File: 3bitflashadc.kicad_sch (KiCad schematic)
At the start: 31 parts, among them U1 LM339, U2 LM339, U3 74148, U4 74LS04, U5 7447

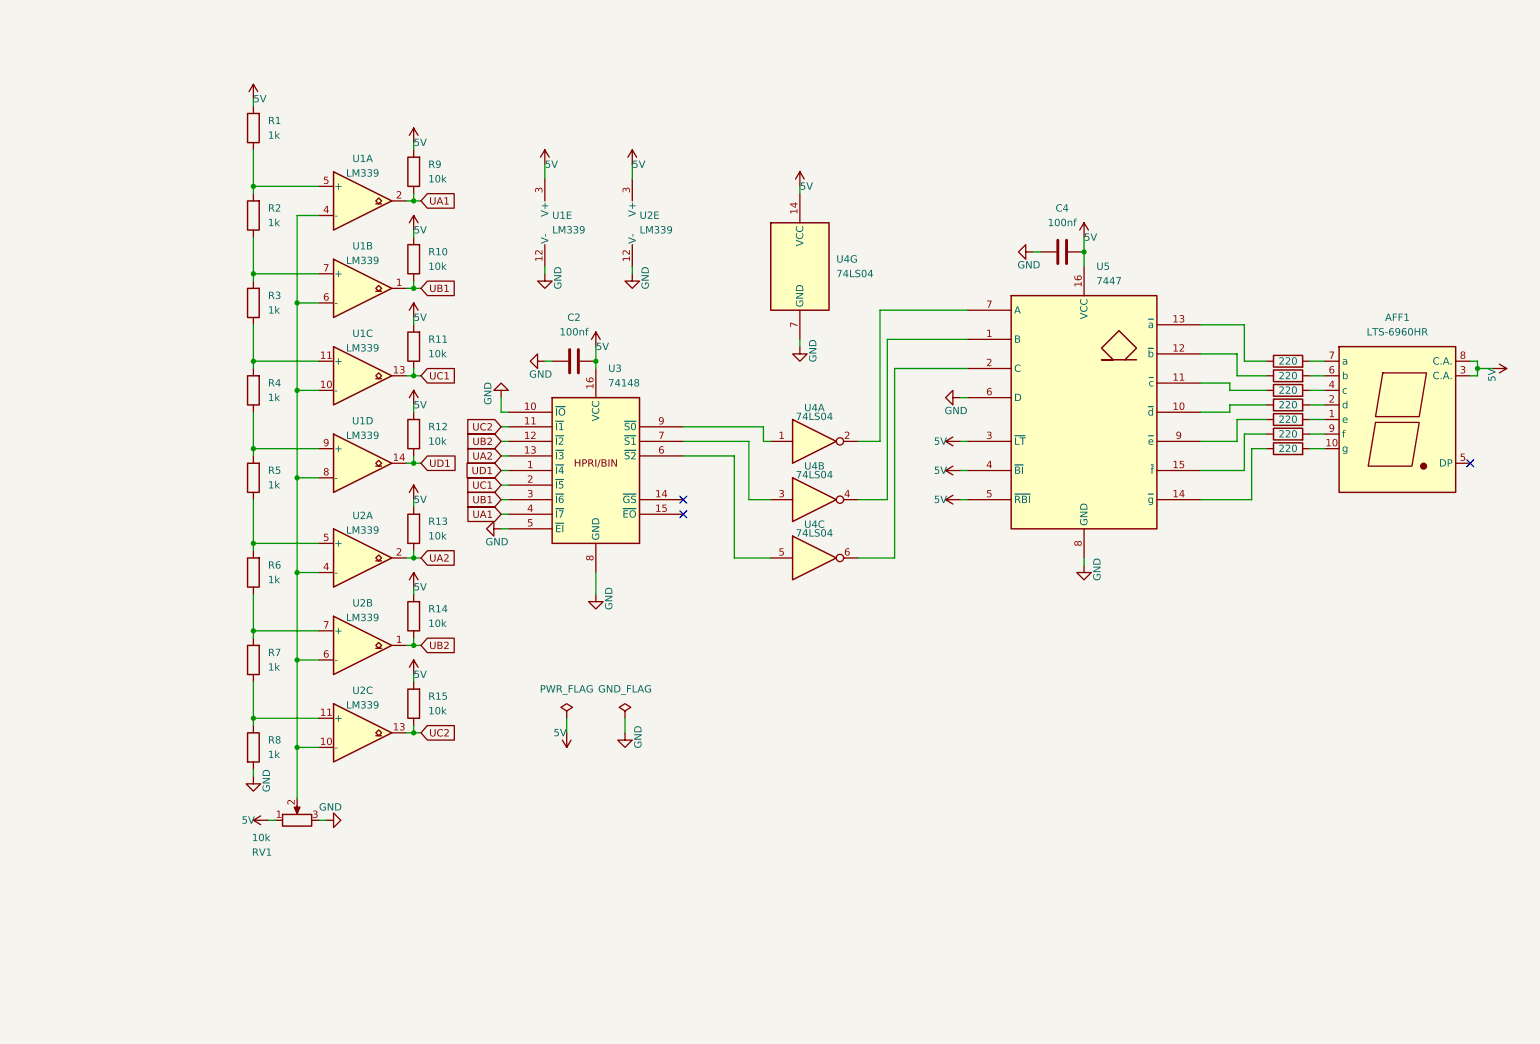
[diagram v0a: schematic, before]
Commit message: Completed schematic, still need to be inspected
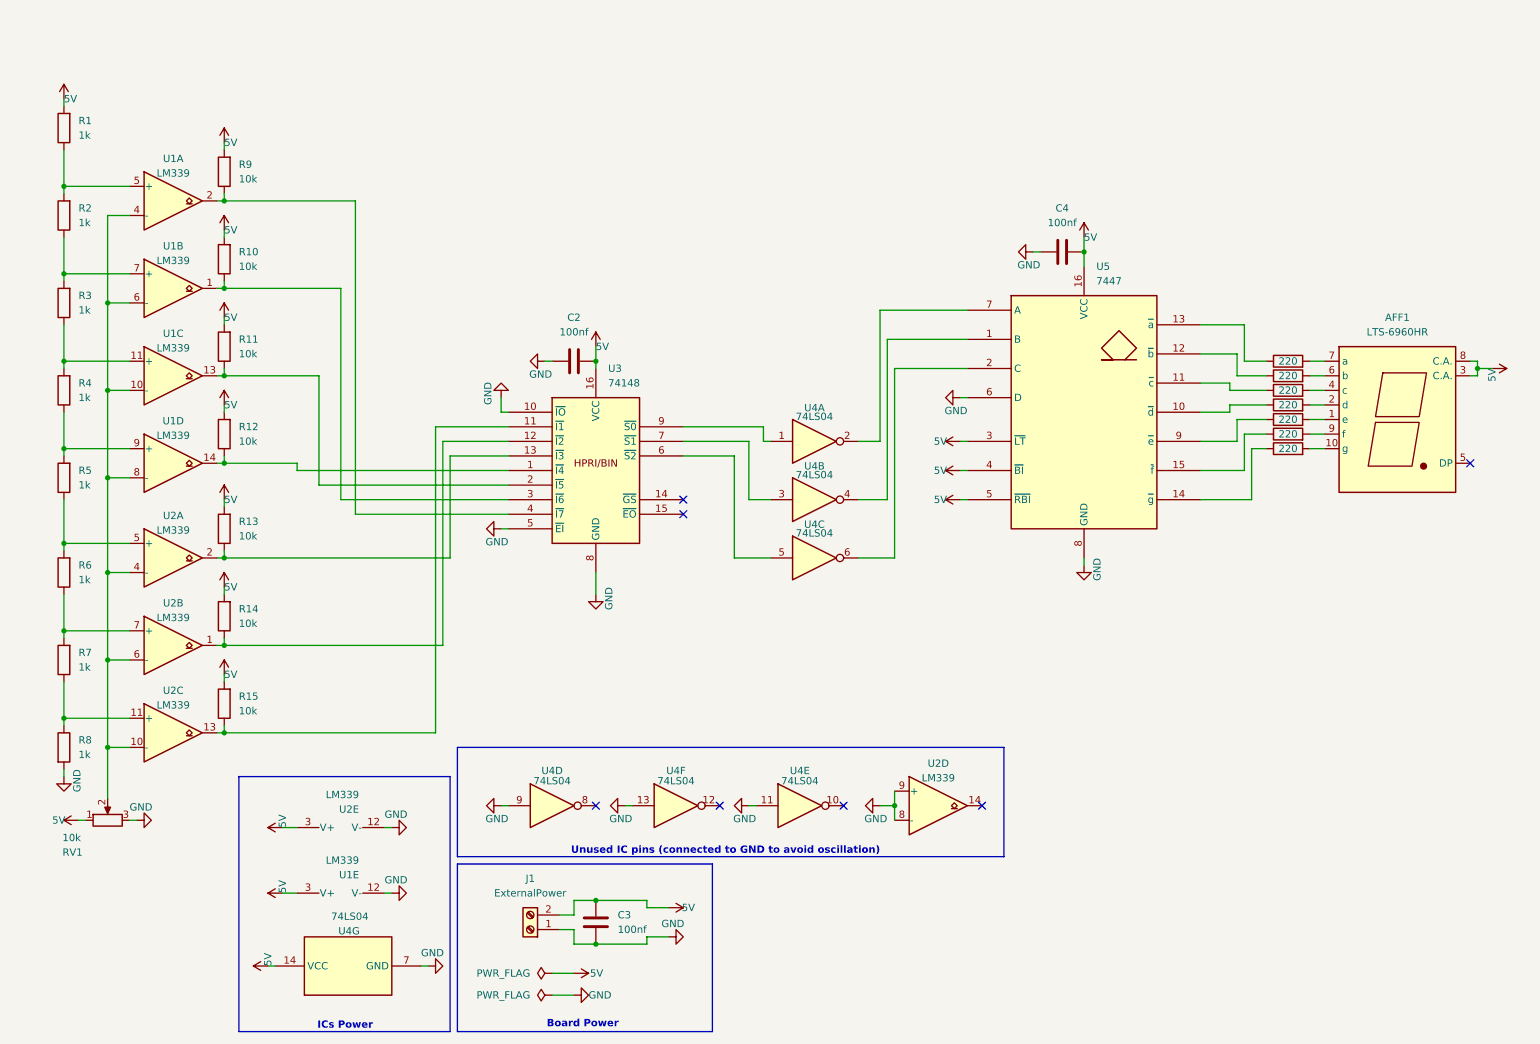
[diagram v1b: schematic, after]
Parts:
- added C3: 100nf, Capacitor_THT:C_Disc_D3.4mm_W2.1mm_P2.50mm, symbol Device:C
- added J1: ExternalPower, TerminalBlock:TerminalBlock_MaiXu_MX126-5.0-02P_1x02_P5.00mm, symbol Connector:Screw_Terminal_01x02
- added unit 4 of U2
- added unit 4 of U4
- added unit 6 of U4
- added unit 5 of U4
- U3: footprint Package_DIP:CERDIP-14_W7.62mm_SideBrazed_LongPads -> Package_DIP:CERDIP-16_W7.62mm_SideBrazed_LongPads
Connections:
- net 5V: now also C3.2, J1.2 (Pin_2)
- net GND: now also C3.1, J1.1 (Pin_1), U2.8 (-), U2.9 (+), U4.11, U4.13, U4.9
- net UA1: no longer names the net of R9.1, U1.2, U3.4 (~{I7})
- net UA2: no longer names the net of R13.1, U2.2, U3.13 (~{I3})
- net UB1: no longer names the net of R10.1, U1.1, U3.3 (~{I6})
- net UB2: no longer names the net of R14.1, U2.1, U3.12 (~{I2})
- net UC1: no longer names the net of R11.1, U1.13, U3.2 (~{I5})
- net UC2: no longer names the net of R15.1, U2.13, U3.11 (~{I1})
- net UD1: no longer names the net of R12.1, U1.14, U3.1 (~{I4})
- no-connect marks 3 -> 7
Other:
- note added: "Board Power"
- note added: "ICs Power"
- note added: "Unused IC pins (connected to GND to avoid oscillation)"
- moved on the sheet: R1, R10, R11, R12, R13, R14, R15, R2, R3, R4, R5, R6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

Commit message: Done with the schematic and working with the PCB routing
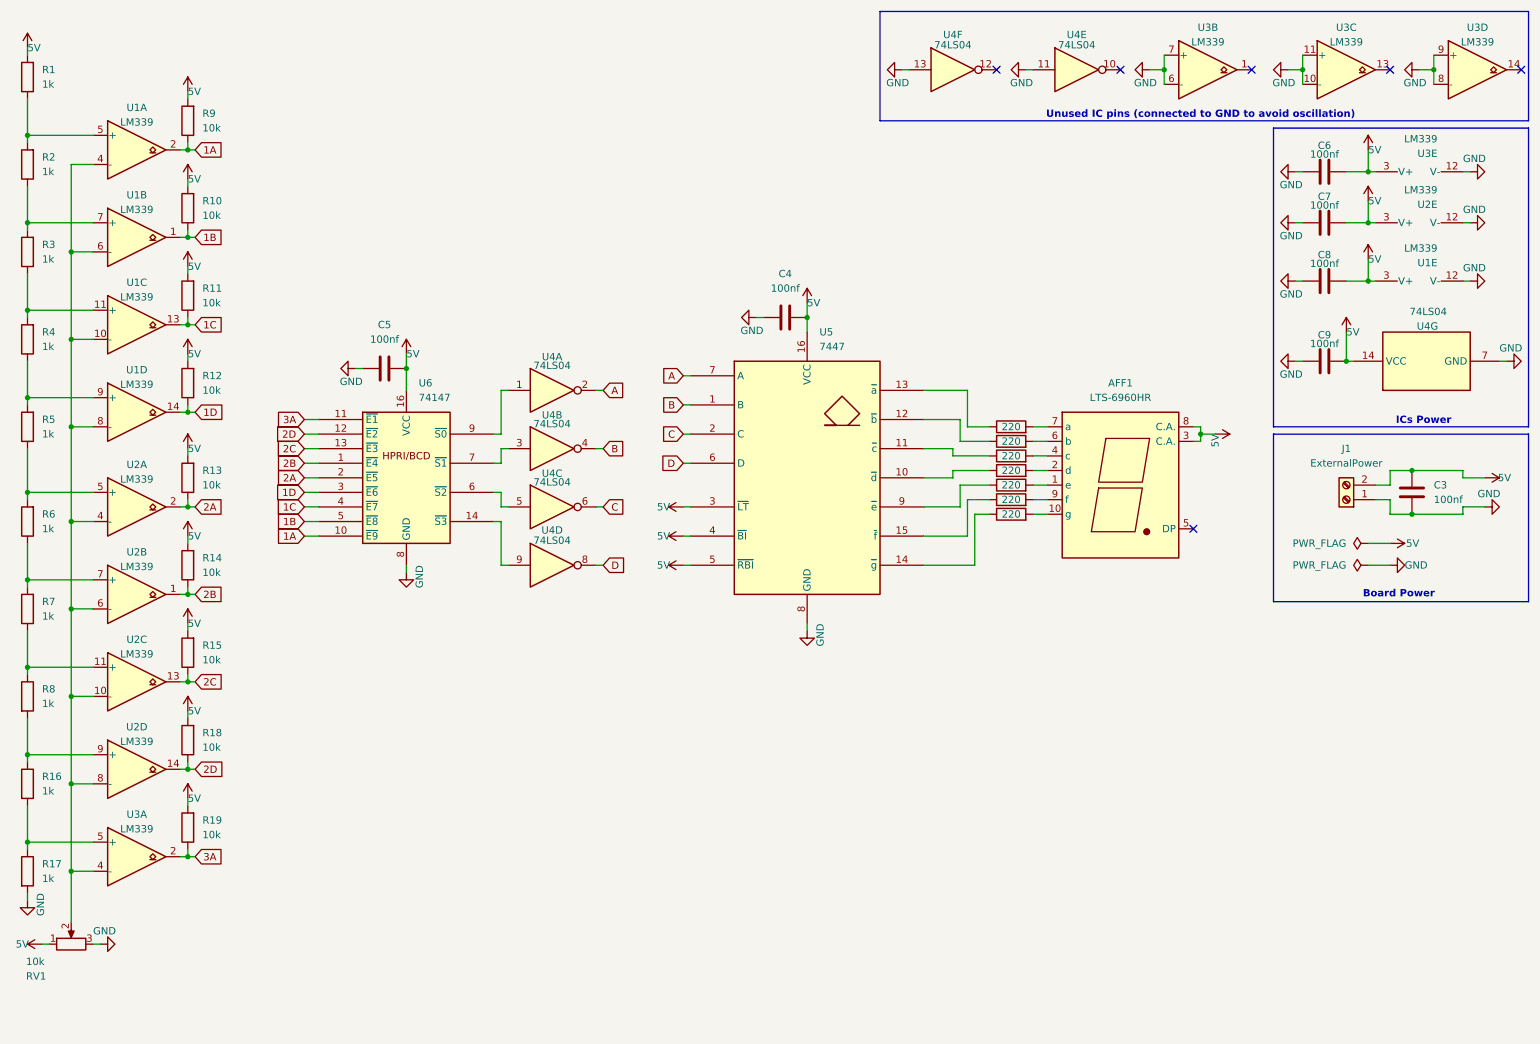
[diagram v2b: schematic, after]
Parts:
- removed C2: 100nf, Capacitor_THT:C_Disc_D3.4mm_W2.1mm_P2.50mm, symbol Device:C
- removed U3: 74148, Package_DIP:CERDIP-16_W7.62mm_SideBrazed_LongPads, symbol 74xx_IEEE:74148
- added C5, C6, C7, C8, C9: 100nf, Capacitor_THT:C_Disc_D3.4mm_W2.1mm_P2.50mm, symbol Device:C
- added R16, R17: 1k, Resistor_THT:R_Axial_DIN0207_L6.3mm_D2.5mm_P7.62mm_Horizontal, symbol Device:R
- added R18, R19: 10k, Resistor_THT:R_Axial_DIN0207_L6.3mm_D2.5mm_P7.62mm_Horizontal, symbol Device:R
- added U3: LM339, Package_DIP:CERDIP-14_W7.62mm_SideBrazed_LongPads_Socket, symbol Comparator:LM339
- added U6: 74147, Package_DIP:CERDIP-16_W7.62mm_SideBrazed_Socket, symbol 74xx_IEEE:74147
- U1, U2, U4: footprint Package_DIP:CERDIP-14_W7.62mm_SideBrazed_LongPads -> Package_DIP:CERDIP-14_W7.62mm_SideBrazed_LongPads_Socket
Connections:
- net 5V: now also C5.2, C6.2, C7.2, C8.2, C9.2, R18.2, R19.2, U3.3 (V+), U6.16 (VCC)
- net GND: now also C5.1, C6.1, C7.1, C8.1, C9.1, R17.2, U3.10 (-), U3.11 (+), U3.12 (V-), U3.6 (-), U3.7 (+), U3.8 (-), U3.9 (+), U6.8 (GND); no longer R8.2, U2.8 (-), U2.9 (+), U4.9, U5.6 (D)
- net 1D: now reaches R12.1, U1.14
- net 1D: now also U6.3 (~{E6})
- net at RV1.2, U1.10 (-), U1.4 (-)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: now also U2.8 (-), U3.4 (-)
- net 2B: now reaches R14.1, U2.1
- net 2B: now also U6.1 (~{E4})
- net at U4.3: now also U6.7 (~{S1})
- net B: now reaches U4.4, U5.1 (B)
- net 1C: now reaches R11.1, U1.13
- net 1C: now also U6.4 (~{E7})
- net 2C: now reaches R15.1, U2.13
- net 2C: now also U6.13 (~{E3})
- net at U4.1: now also U6.9 (~{S0})
- net A: now reaches U4.2, U5.7 (A)
- net 2D: now reaches U2.14
- net 2D: now also R18.1, U6.12 (~{E2})
- net D: now reaches U4.8
- net D: now also U5.6 (D)
- net 2A: now reaches R13.1, U2.2
- net 2A: now also U6.2 (~{E5})
- net 1B: now reaches R10.1, U1.1
- net 1B: now also U6.5 (~{E8})
- net C: now reaches U4.6, U5.2 (C)
- net 1A: now reaches R9.1, U1.2
- net 1A: now also U6.10 (~{E9})
- net at U4.5: now also U6.6 (~{S2})
- new net: R16.1, R8.2, U2.9 (+)
- new net: U4.9, U6.14 (~{S3})
- new net: R16.2, R17.1, U3.5 (+)
- new net 3A: R19.1, U3.2, U6.11 (~{E1})
- no-connect marks 7 -> 6
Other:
- moved on the sheet: AFF1, C3, C4, J1, R1, R10, R11, R12, R13, R14, R15, R2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
